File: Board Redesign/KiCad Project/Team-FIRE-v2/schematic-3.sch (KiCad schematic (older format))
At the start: 14 parts, among them IC2 BTS500601TEAAUMA2, U8 TPS82140SILR

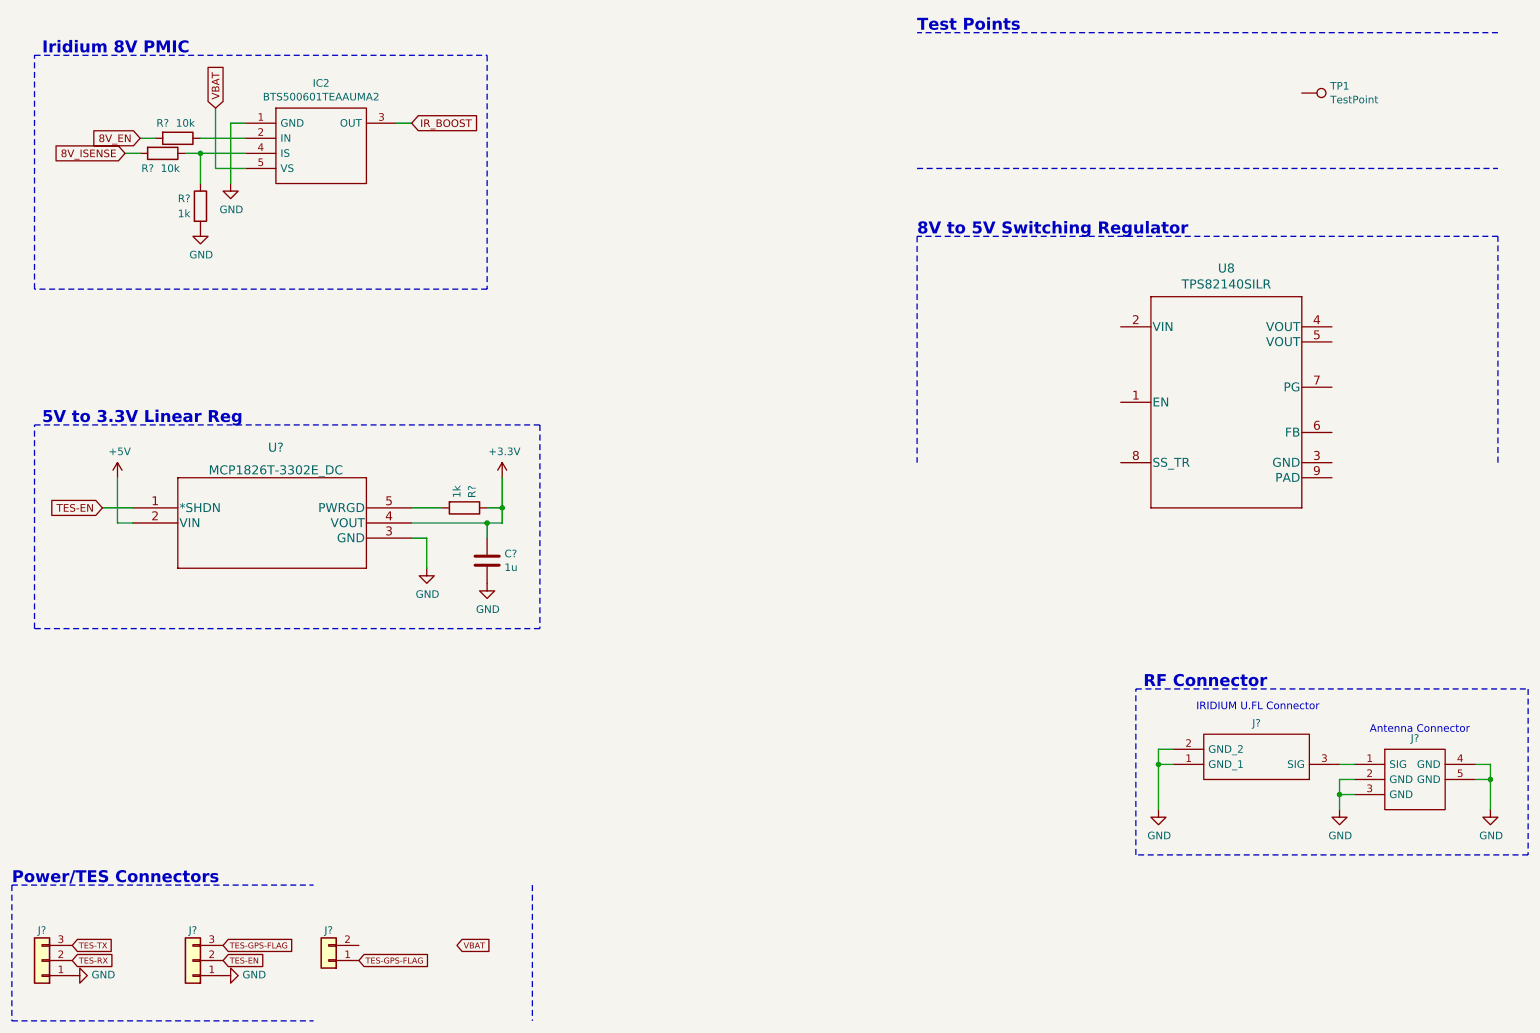
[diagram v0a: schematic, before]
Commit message: Buck Converter & Test Points
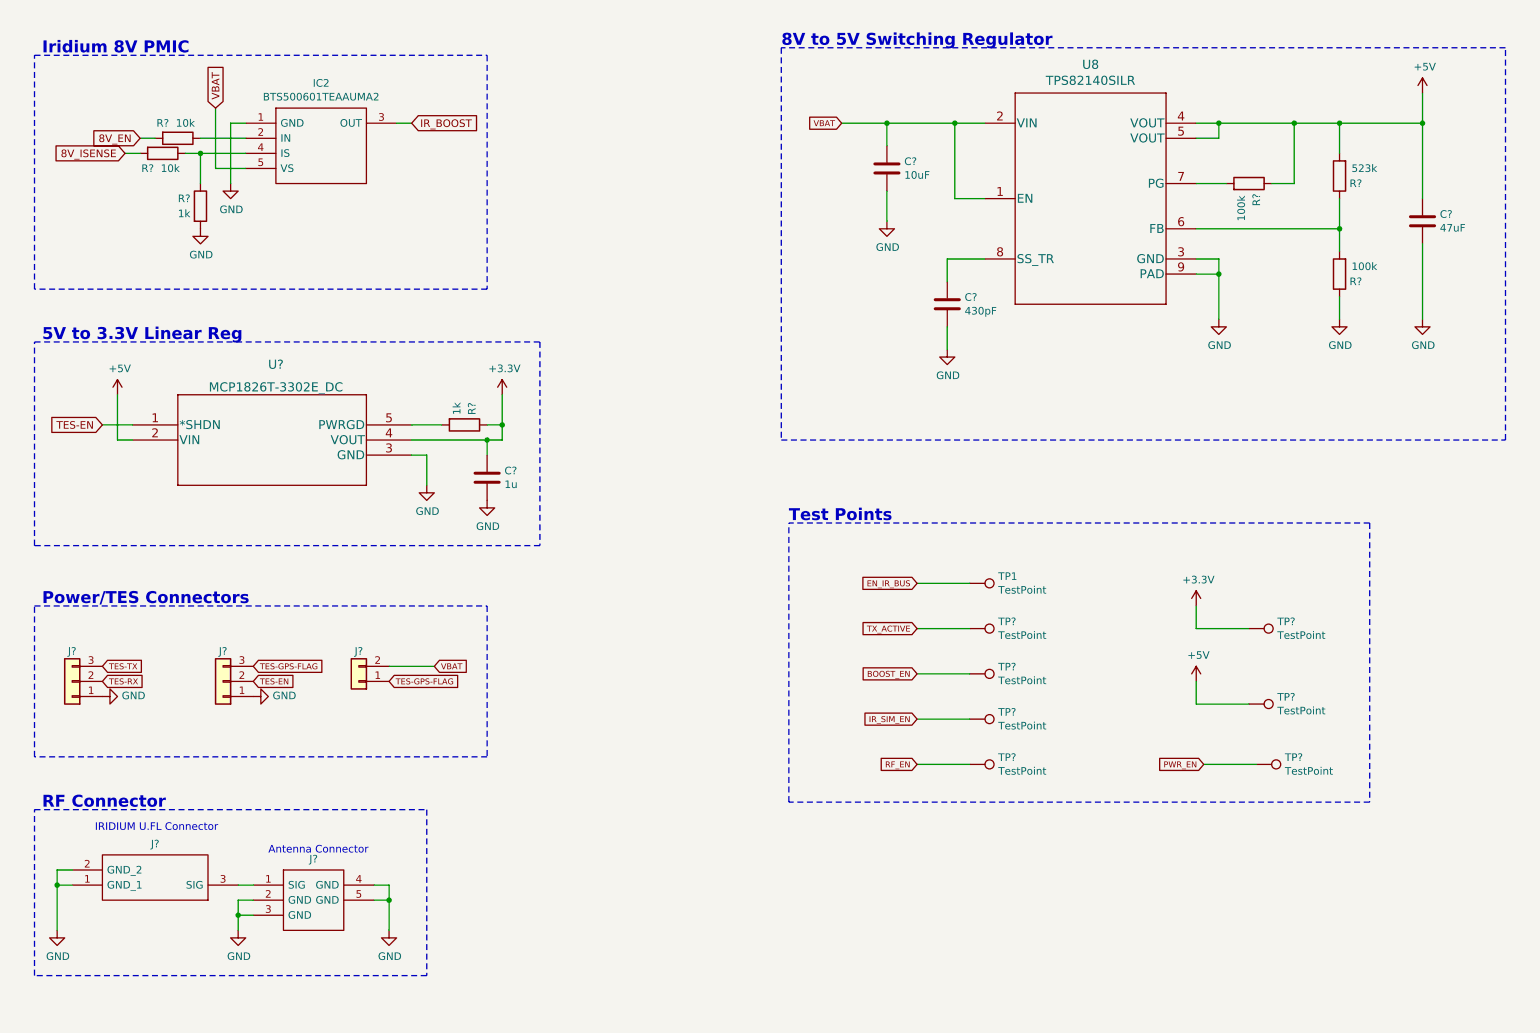
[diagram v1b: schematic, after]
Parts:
- added C?: 10uF, Capacitor_SMD:C_0805_2012Metric, symbol Device:C
- added C?: 430pF, Capacitor_SMD:C_0805_2012Metric, symbol Device:C
- added C?: 47uF, Capacitor_SMD:C_0805_2012Metric, symbol Device:C
- added R? (x2): 100k, Resistor_SMD:R_0603_1608Metric, symbol Device:R
- added R?: 523k, Resistor_SMD:R_0603_1608Metric, symbol Device:R
- added TP? (x7): TestPoint, symbol Connector:TestPoint
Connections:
- net +3V3: now also TP?.1
- net +5V: now also U8.4 (VOUT), U8.5 (VOUT), C?.1, R?.1, R?.2, TP?.1
- net GND: now also U8.3 (GND), U8.9 (PAD), C?.2, C?.2, C?.2, R?.1
- net VBAT: now also J?.2 (Pin_2), U8.1 (EN), U8.2 (VIN), C?.1
- net EN_IR_BUS: now reaches TP1.1
- net at U8.6 (FB): now also R?.1, R?.2
- net at U8.7 (PG): now also R?.2
- net at U8.8 (SS_TR): now also C?.1
- new net BOOST_EN: TP?.1
- new net IR_SIM_EN: TP?.1
- new net PWR_EN: TP?.1
- new net RF_EN: TP?.1
- new net TX_ACTIVE: TP?.1
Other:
- moved on the sheet: C?, J?, R?, TP1, U8, U?
